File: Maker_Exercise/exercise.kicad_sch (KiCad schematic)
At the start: 13 parts, among them J1 USB_C_Receptacle_USB2.0_16P, U1 USBLC6-2SC6, U2 STM32G431CBUx

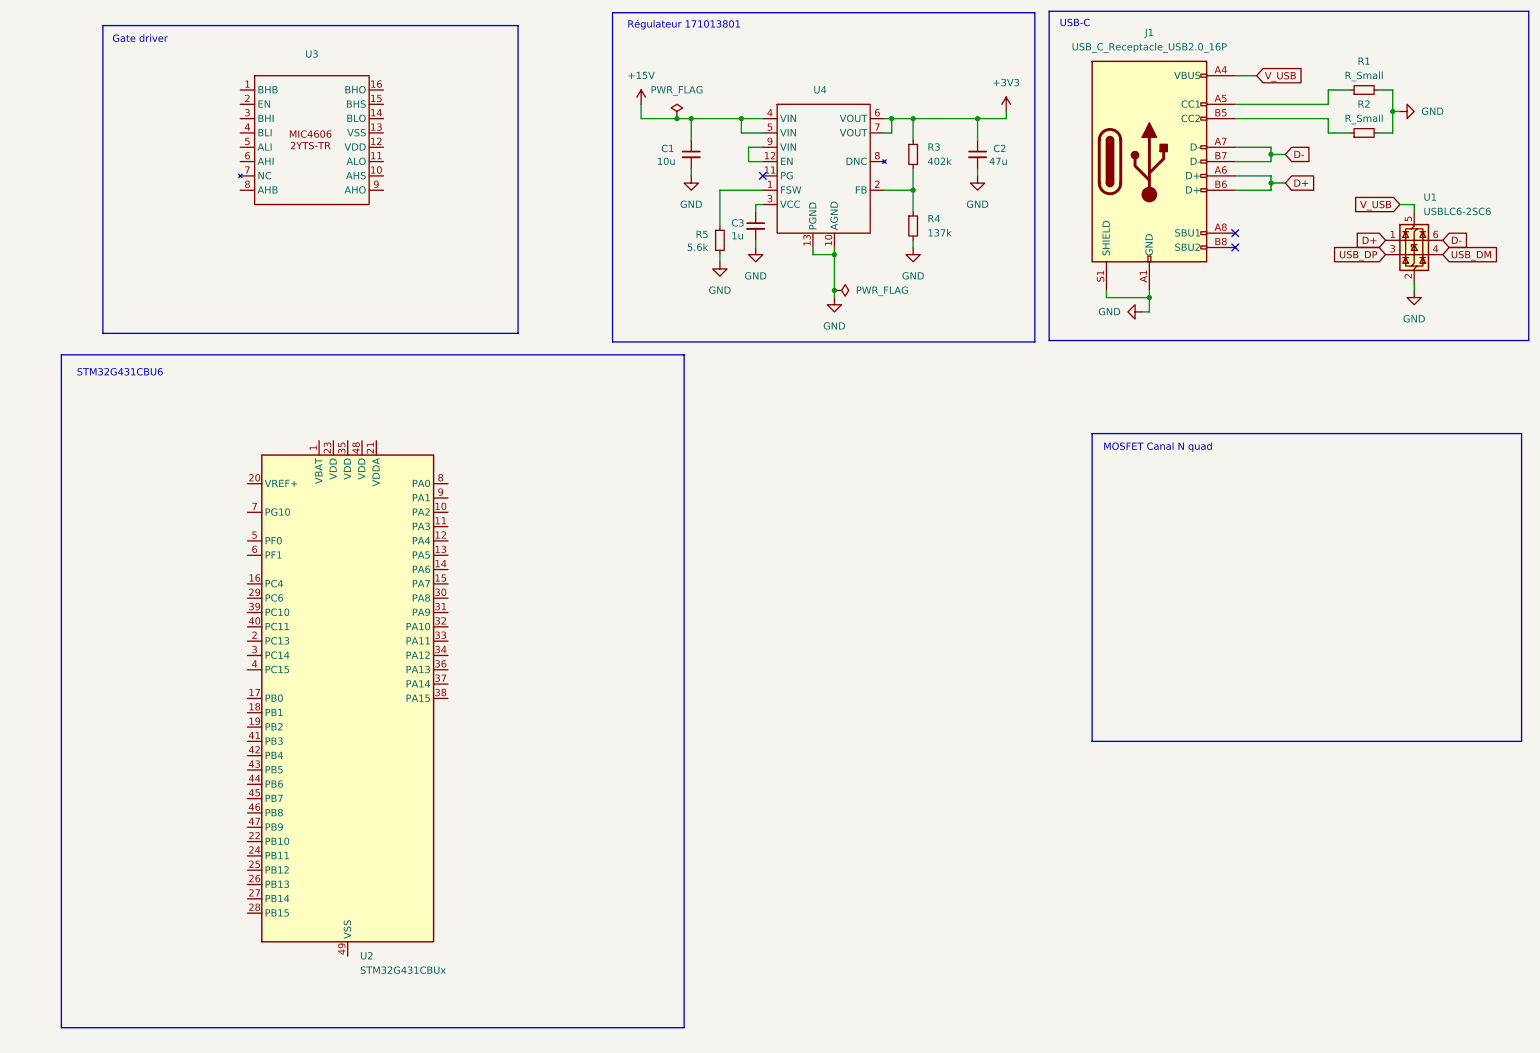
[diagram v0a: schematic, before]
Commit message: Updated schematic
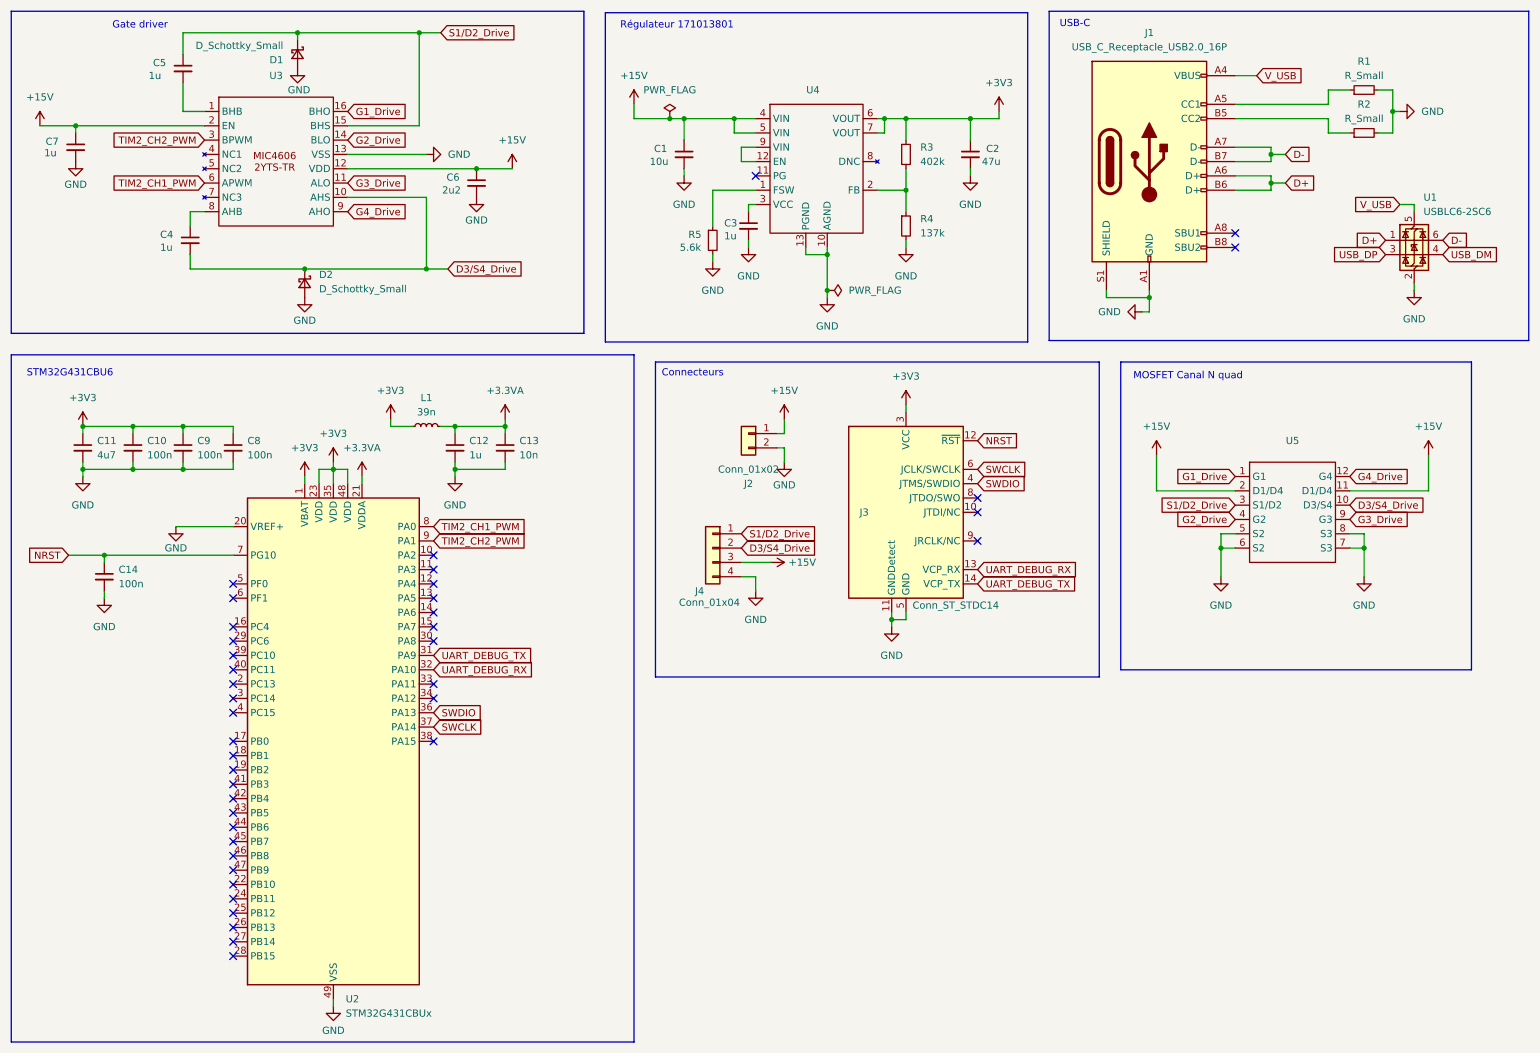
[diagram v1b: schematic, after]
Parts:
- added C10, C14, C8, C9: 100n, symbol Device:C_Small
- added C11: 4u7, symbol Device:C_Small
- added C12, C4, C5, C7: 1u, symbol Device:C_Small
- added C13: 10n, symbol Device:C_Small
- added C6: 2u2, symbol Device:C_Small
- added D1, D2: D_Schottky_Small, symbol Device:D_Schottky_Small
- added J2: Conn_01x02, symbol Connector_Generic:Conn_01x02
- added J3: Conn_ST_STDC14, symbol Connector:Conn_ST_STDC14
- added J4: Conn_01x04, symbol Connector_Generic:Conn_01x04
- added L1: 39n, symbol Device:L_Small
- added U5: ~, symbol maker:FDMQ86530L
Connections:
- net +15V: now also U3.12 (VDD), U3.2 (EN), C6.1, C7.1, J2.1 (Pin_1), J4.3 (Pin_3), U5.11 (D1/D4), U5.2 (D1/D4)
- net +3V3: now also U2.1 (VBAT), U2.23 (VDD), U2.35 (VDD), U2.48 (VDD), C10.1, C11.1, C8.1, C9.1, J3.3 (VCC), L1.1
- net GND: now also U2.20 (VREF+), U2.49 (VSS), U3.13 (VSS), C10.2, C11.2, C12.2, C13.2, C14.2, C6.2, C7.2, C8.2, C9.2, D1.2 (A), D2.2 (A), J2.2 (Pin_2), J3.11 (GNDDetect), J3.5 (GND), J3.7 (GND), J4.4 (Pin_4), U5.5 (S2), U5.6 (S2), U5.7 (S3), U5.8 (S3)
- net +3.3VA: now reaches U2.21 (VDDA)
- net +3.3VA: now also C12.1, C13.1, L1.2
- net UART_DEBUG_TX: now reaches U2.31 (PA9)
- net UART_DEBUG_TX: now also J3.14 (VCP_TX)
- net UART_DEBUG_RX: now reaches U2.32 (PA10)
- net UART_DEBUG_RX: now also J3.13 (VCP_RX)
- net SWDIO: now reaches U2.36 (PA13)
- net SWDIO: now also J3.4 (JTMS/SWDIO)
- net SWCLK: now reaches U2.37 (PA14)
- net SWCLK: now also J3.6 (JCLK/SWCLK)
- net NRST: now reaches U2.7 (PG10)
- net NRST: now also C14.1, J3.12 (~{RST})
- net TIM2_CH1_PWM: now reaches U2.8 (PA0)
- net TIM2_CH1_PWM: now also U3.6 (APWM)
- net TIM2_CH2_PWM: now reaches U2.9 (PA1)
- net TIM2_CH2_PWM: now also U3.3 (BPWM)
- net at U3.1 (BHB): now also C5.2
- net D3/S4_Drive: now reaches U3.10 (AHS)
- net D3/S4_Drive: now also C4.2, D2.1 (K), J4.2 (Pin_2), U5.10 (D3/S4)
- net G3_Drive: now reaches U3.11 (ALO)
- net G3_Drive: now also U5.9 (G3)
- net G2_Drive: now reaches U3.14 (BLO)
- net G2_Drive: now also U5.4 (G2)
- net S1/D2_Drive: now reaches U3.15 (BHS)
- net S1/D2_Drive: now also C5.1, D1.1 (K), J4.1 (Pin_1), U5.3 (S1/D2)
- net G1_Drive: now reaches U3.16 (BHO)
- net G1_Drive: now also U5.1 (G1)
- net at U3.8 (AHB): now also C4.1
- net G4_Drive: now reaches U3.9 (AHO)
- net G4_Drive: now also U5.12 (G4)
- no-connect marks 3 -> 41
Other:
- note added: "Connecteurs"
- company: (none) -> ENSEA
- title: (none) -> Maker_Exercise
- moved on the sheet: C1, C2, C3, R3, R4, R5, U2, U4
